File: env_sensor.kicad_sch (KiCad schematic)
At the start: 30 parts, among them J1 E Paper, J10 Conn_01x06_Pin, J2 5V_in, J3 Barrel_Jack, J4 LED_OUTPUT, J5 Conn_01x02_Pin, J6 Conn_01x04_Socket, J7 Conn_01x04_Socket, J8 v5_v3, J9 v5_v12, Q1 NMOS, Q2 NMOS, Q3 NMOS, U1 ESP32-DevKitC, U1 MH-Z19B, U3 DRV8847SPWR, U4 TXB0104PW, U5 BME280

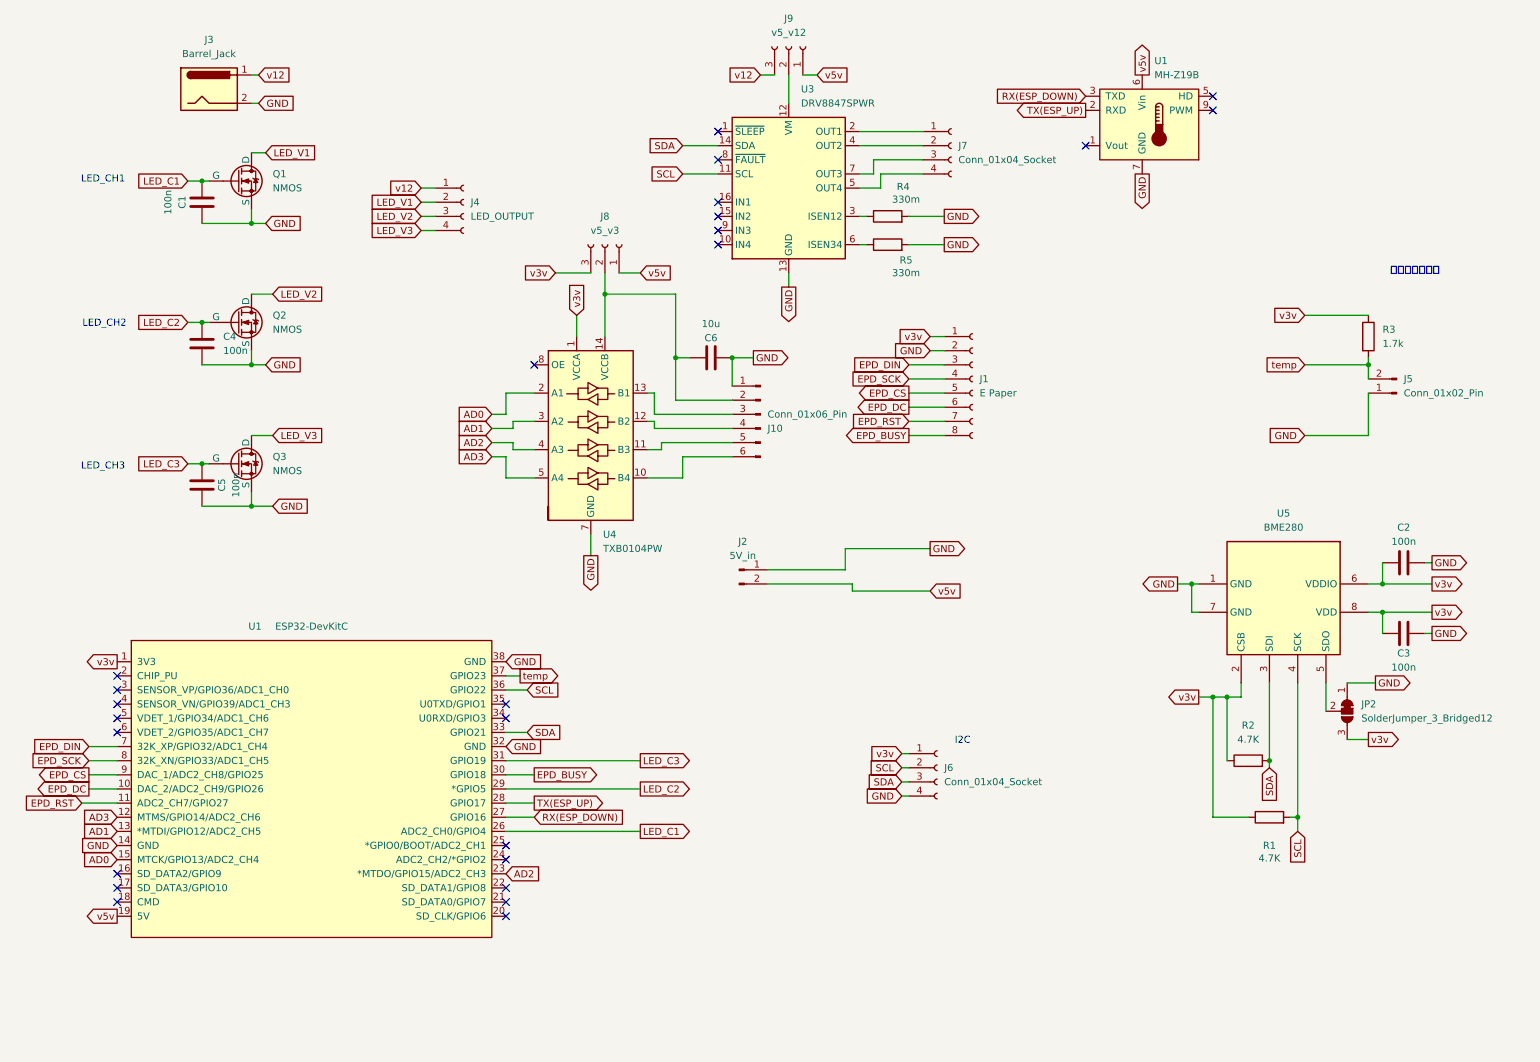
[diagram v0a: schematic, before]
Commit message: update pcb
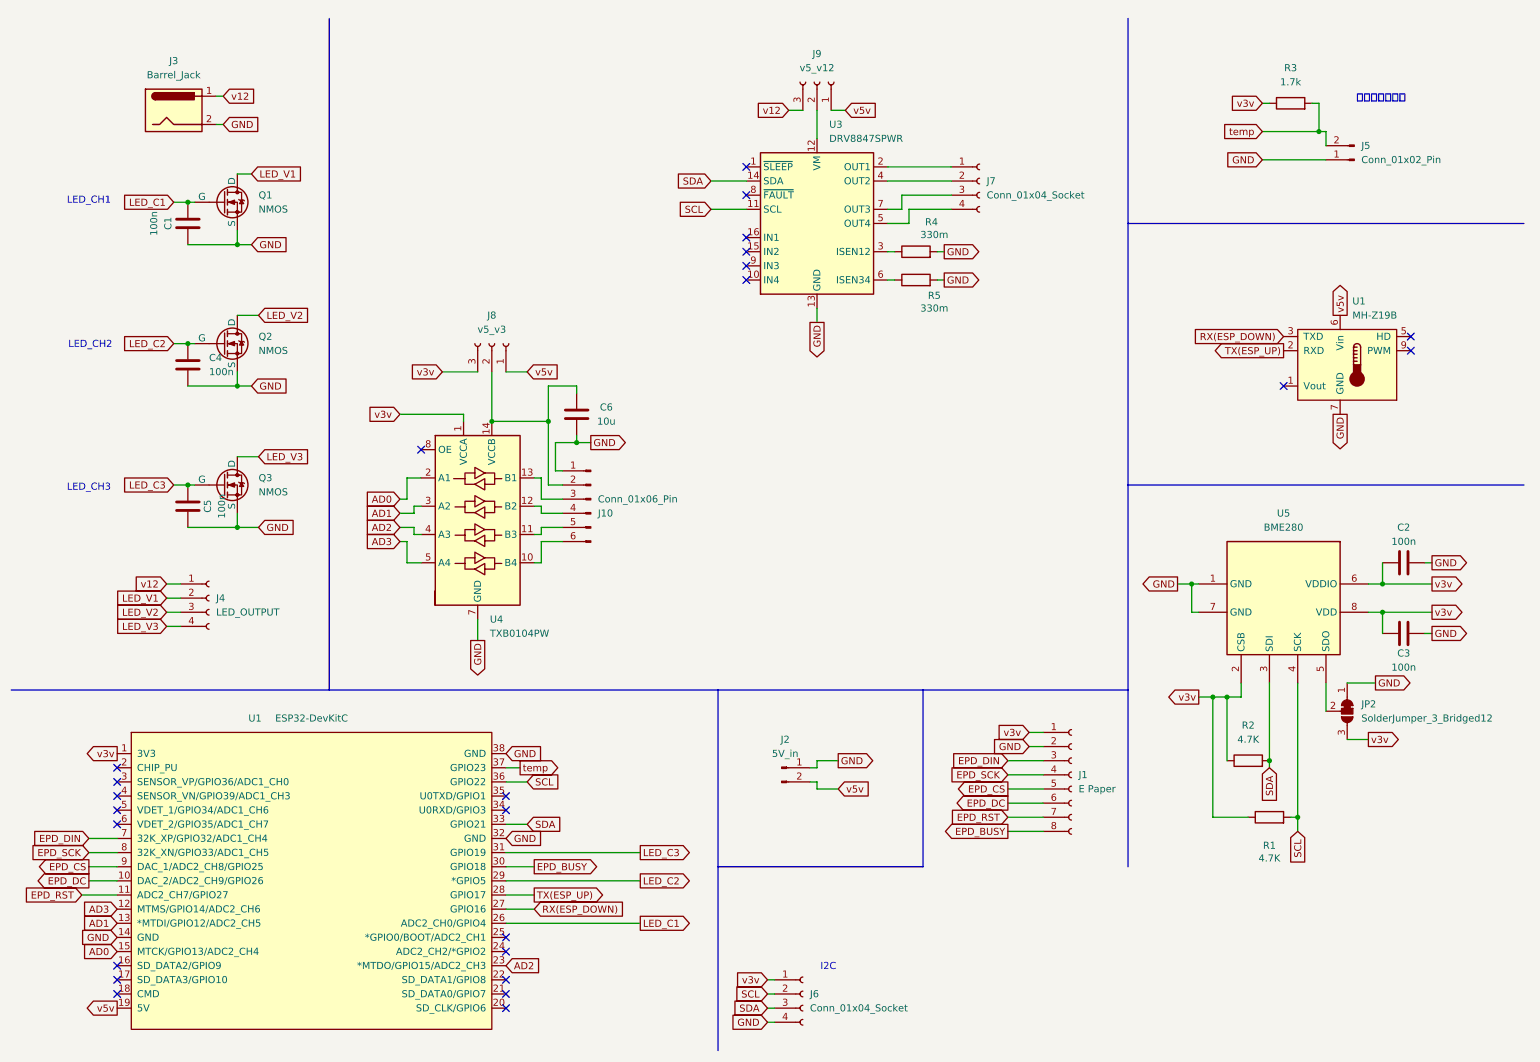
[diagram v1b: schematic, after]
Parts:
- C6: LCSC C141660 -> C267437
- R1, R2: LCSC C23164 -> C99782
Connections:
- net GND: now also C6.2; no longer C6.1
- net at J10.2 (Pin_2), J8.2 (Pin_2), U4.14 (VCCB): now also C6.1; no longer C6.2
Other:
- moved on the sheet: C1, C4, C5, C6, J1, J10, J2, J3, J4, J5, J6, J7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

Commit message: update bom
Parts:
- C6: LCSC C267437 -> C466783
- J1, J2, J3, J4, J5, J6, J7, J8, J9, U1: now left out of the parts list
- R1, R2: LCSC C99782 -> C23162
- R3: LCSC C863146 -> C22936
- R4, R5: LCSC (none) -> C22978
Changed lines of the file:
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@@
 			)
 		)
-		(property "LCSC" "C267437"
+		(property "LCSC" "C466783"
 			(at 114.3 83.82 90)
 			(effects
@@
 		(unit 1)
 		(exclude_from_sim no)
-		(in_bom yes)
-		(on_board yes)
+		(in_bom no)
+		(on_board no)
 		(dnp no)
 		(fields_autoplaced yes)
@@
 		(unit 1)
 		(exclude_from_sim no)
-		(in_bom yes)
-		(on_board yes)
+		(in_bom no)
+		(on_board no)
 		(dnp no)
 		(fields_autoplaced yes)
@@
 		(unit 1)
 		(exclude_from_sim no)
-		(in_bom yes)
-		(on_board yes)
+		(in_bom no)
+		(on_board no)
 		(dnp no)
 		(fields_autoplaced yes)
@@
 			)
 		)
+		(property "LCSC" "C22978"
+			(at 175.26 54.61 90)
+			(effects
+				(font
+					(size 1.27 1.27)
+				)
+				(hide yes)
+			)
+		)
 		(pin "1"
 		)
@@
 			)
 		)
-		(property "LCSC" "C99782"
+		(property "LCSC" "C23162"
 			(at 238.76 156.21 0)
 			(effects
@@
 			)
 		)
-		(property "LCSC" "C863146"
+		(property "LCSC" "C22936"
 			(at 242.57 27.94 0)
 			(effects
@@
 		(unit 1)
 		(exclude_from_sim no)
-		(in_bom yes)
-		(on_board yes)
+		(in_bom no)
+		(on_board no)
 		(dnp no)
 		(property "Reference" "J8"
@@
 		(unit 1)
 		(exclude_from_sim no)
-		(in_bom yes)
-		(on_board yes)
+		(in_bom no)
+		(on_board no)
 		(dnp no)
 		(property "Reference" "J9"
@@
 		(unit 1)
 		(exclude_from_sim no)
-		(in_bom yes)
-		(on_board yes)
+		(in_bom no)
+		(on_board no)
 		(dnp no)
 		(property "Reference" "U1"
@@
 			)
 		)
-		(property "LCSC" "C99782"
+		(property "LCSC" "C23162"
 			(at 234.95 146.05 0)
 			(effects
@@
 		(unit 1)
 		(exclude_from_sim no)
-		(in_bom yes)
-		(on_board yes)
+		(in_bom no)
+		(on_board no)
 		(dnp no)
 		(fields_autoplaced yes)
@@
 		(unit 1)
 		(exclude_from_sim no)
-		(in_bom yes)
-		(on_board yes)
+		(in_bom no)
+		(on_board no)
 		(dnp no)
 		(fields_autoplaced yes)
@@
 			)
 		)
+		(property "LCSC" "C22978"
+			(at 175.26 59.69 90)
+			(effects
+				(font
+					(size 1.27 1.27)
+				)
+				(hide yes)
+			)
+		)
 		(pin "1"
 		)
@@
 		(unit 1)
 		(exclude_from_sim no)
-		(in_bom yes)
-		(on_board yes)
+		(in_bom no)
+		(on_board no)
 		(dnp no)
 		(fields_autoplaced yes)
@@
 		(unit 1)
 		(exclude_from_sim no)
-		(in_bom yes)
-		(on_board yes)
+		(in_bom no)
+		(on_board no)
 		(dnp no)
 		(fields_autoplaced yes)
@@
 		(unit 1)
 		(exclude_from_sim no)
-		(in_bom yes)
-		(on_board yes)
+		(in_bom no)
+		(on_board no)
 		(dnp no)
 		(fields_autoplaced yes)
